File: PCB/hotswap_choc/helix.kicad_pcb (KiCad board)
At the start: 2 copper layers, 135.2 x 94 mm, 134 parts, among them J1 MJ-4PP-9, P1 CONN_01X01, P2 CONN_01X01, P3 OLED, P4 LED, SW1 SW_PUSH, SW10 SW_PUSH, SW11 SW_PUSH, SW12 SW_PUSH, SW13 SW_PUSH, SW14 SW_PUSH, SW15 SW_PUSH, SW16 SW_PUSH, SW17 SW_PUSH, SW18 SW_PUSH, SW19 SW_PUSH, SW2 SW_PUSH, SW20 SW_PUSH, SW21 SW_PUSH, SW22 SW_PUSH, SW23 SW_PUSH, SW24 SW_PUSH, SW25 SW_PUSH, SW26 SW_PUSH, SW27 SW_PUSH, SW28 SW_PUSH, SW29 SW_PUSH, SW3 SW_PUSH, SW30 SW_PUSH, SW31 SW_PUSH, SW32 SW_PUSH, SW33 Reset, SW4 SW_PUSH, SW5 SW_PUSH, SW6 SW_PUSH, SW7 SW_PUSH, SW8 SW_PUSH, SW9 SW_PUSH, U1 ProMicro, U10 SK6812mini, U11 SK6812mini, U12 SK6812mini, U13 SK6812mini, U14 SK6812mini, U15 SK6812mini, U16 SK6812mini, U17 SK6812mini, U18 SK6812mini, U19 SK6812mini, U2 SK6812mini, U20 SK6812mini, U21 SK6812mini, U22 SK6812mini, U23 SK6812mini, U24 SK6812mini, U25 SK6812mini, U26 SK6812mini, U27 SK6812mini, U28 SK6812mini, U29 SK6812mini, U3 SK6812mini, U30 SK6812mini, U31 SK6812mini, U32 SK6812mini, U33 SK6812mini, U4 SK6812mini, U5 SK6812mini, U6 SK6812mini, U7 SK6812mini, U8 SK6812mini, U9 SK6812mini

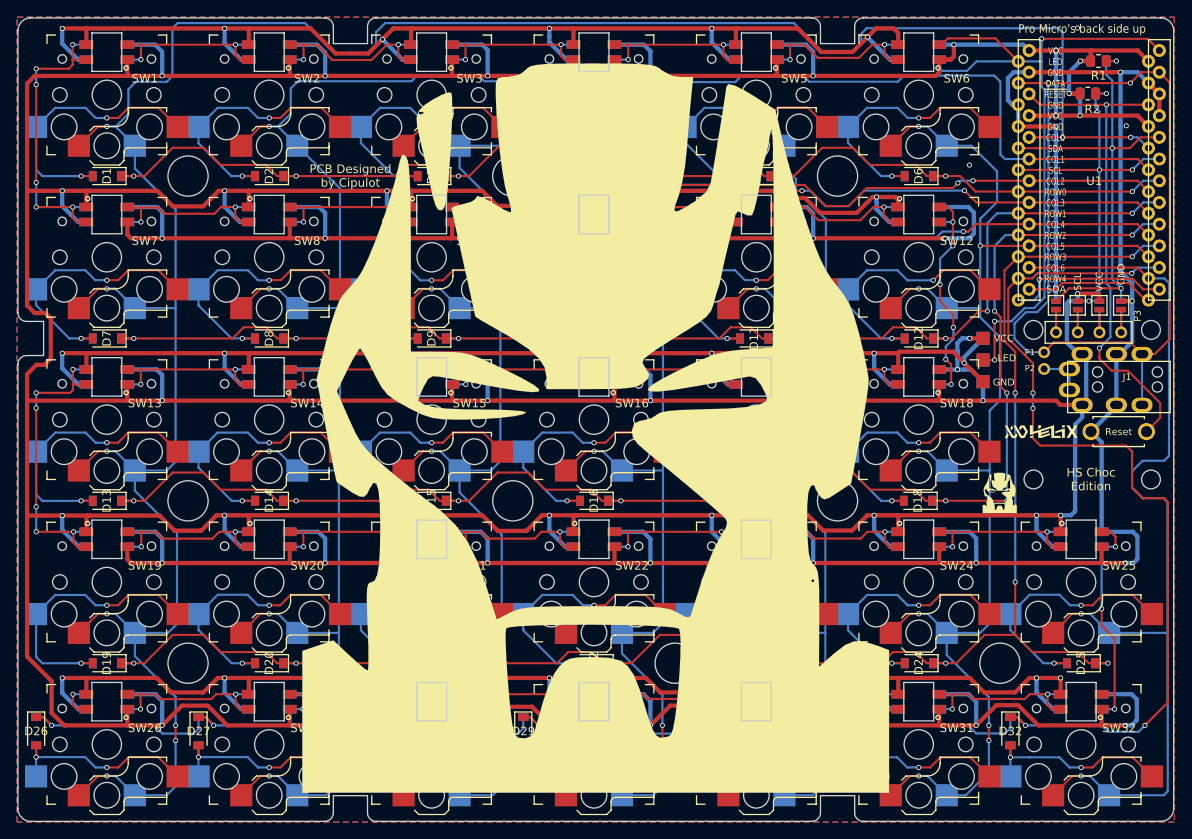
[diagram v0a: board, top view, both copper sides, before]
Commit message: Update
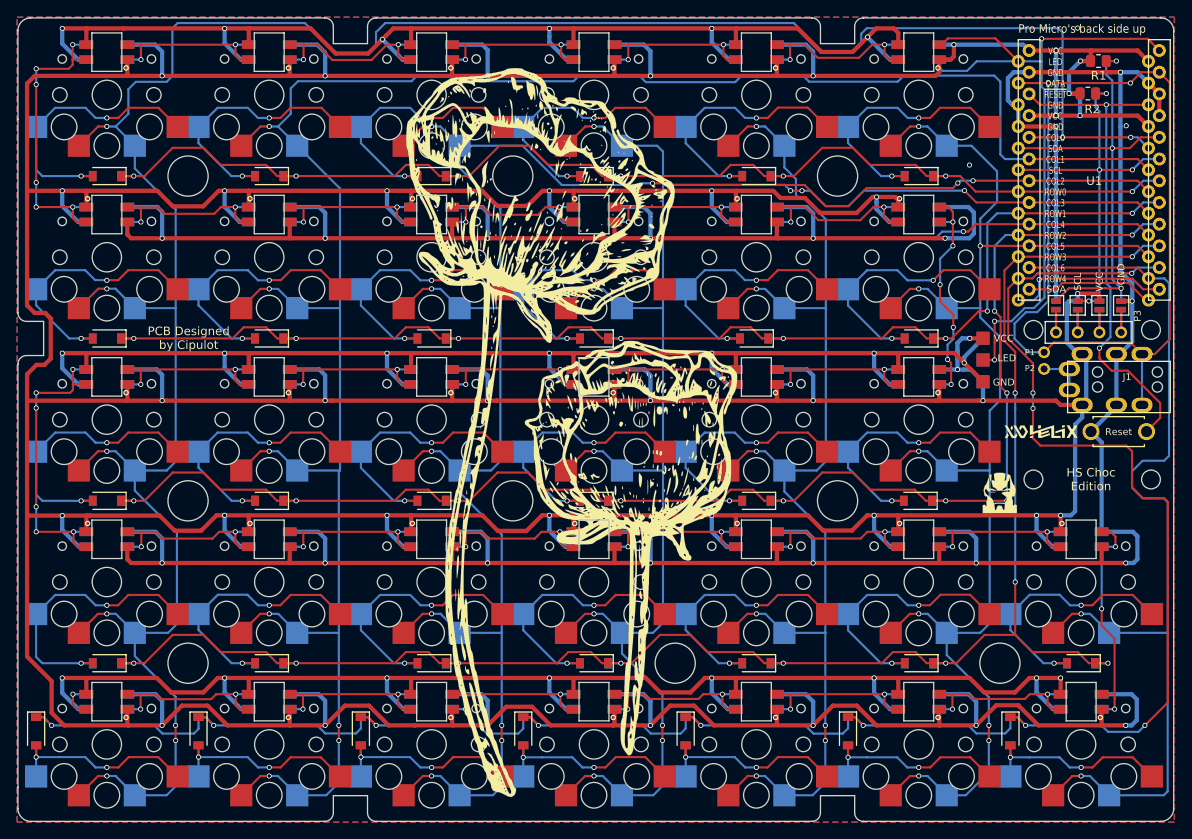
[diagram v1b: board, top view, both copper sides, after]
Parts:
- removed the G*** at (149.0, 91.0)
- added G***: LOGO, Logos:Double_flower_helix, F.Cu at (146.7, 92.2)
- SW1, SW10, SW11, SW12, SW13, SW14, SW15, SW16, SW17, SW18, SW19, SW2, SW20, SW21, SW22, SW23, SW24, SW25, SW26, SW27, SW28, SW29, SW3, SW30, SW31, SW32, SW4, SW5, SW6, SW7, SW8, SW9: footprint Keyswitches:Kailh_socket_PG1350_reversible_LEFT -> Keyswitches:Kailh_socket_PG1350_reversible_LEFT_nosilkangle
